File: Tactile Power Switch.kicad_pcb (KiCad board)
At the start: 2 copper layers, 24 x 30 mm, 16 parts, among them J1 OSTTC020162, J2 OSTTC020162, Q1 BC847B_215, Q2 BC847B_215, Q4 NDT2955

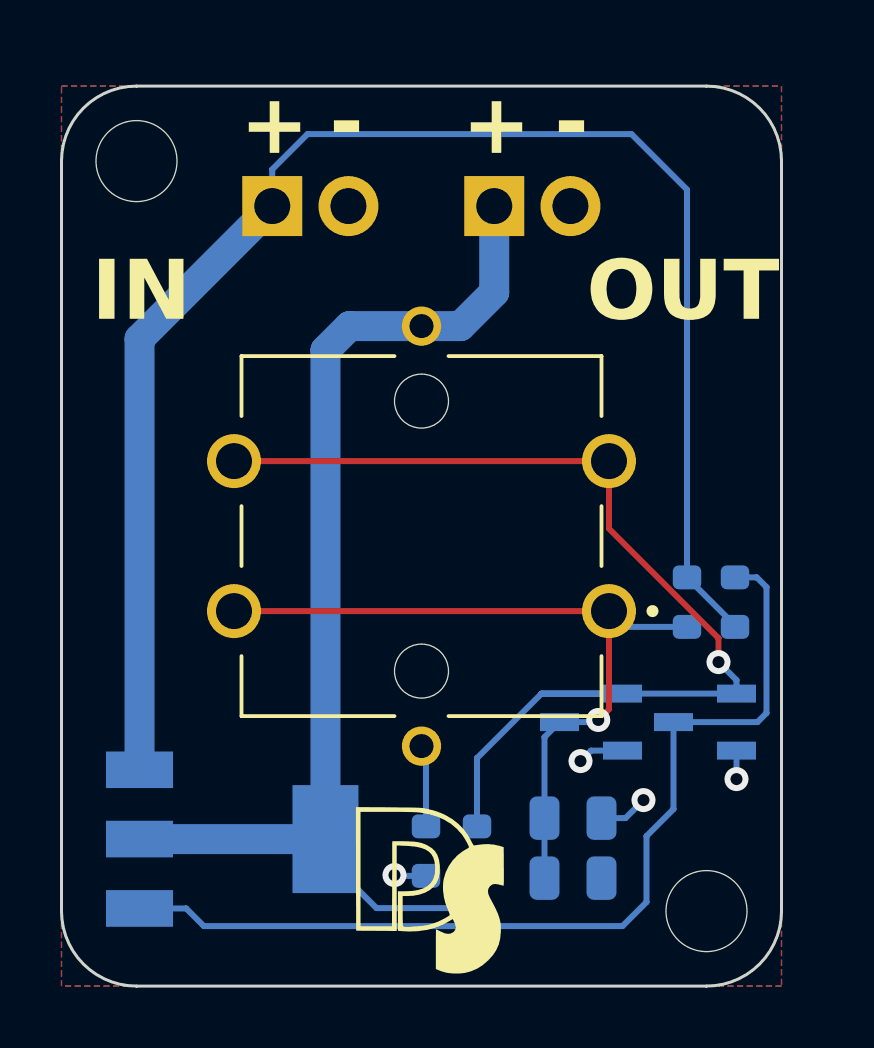
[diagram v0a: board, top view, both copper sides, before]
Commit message: SMD version: Placement is done
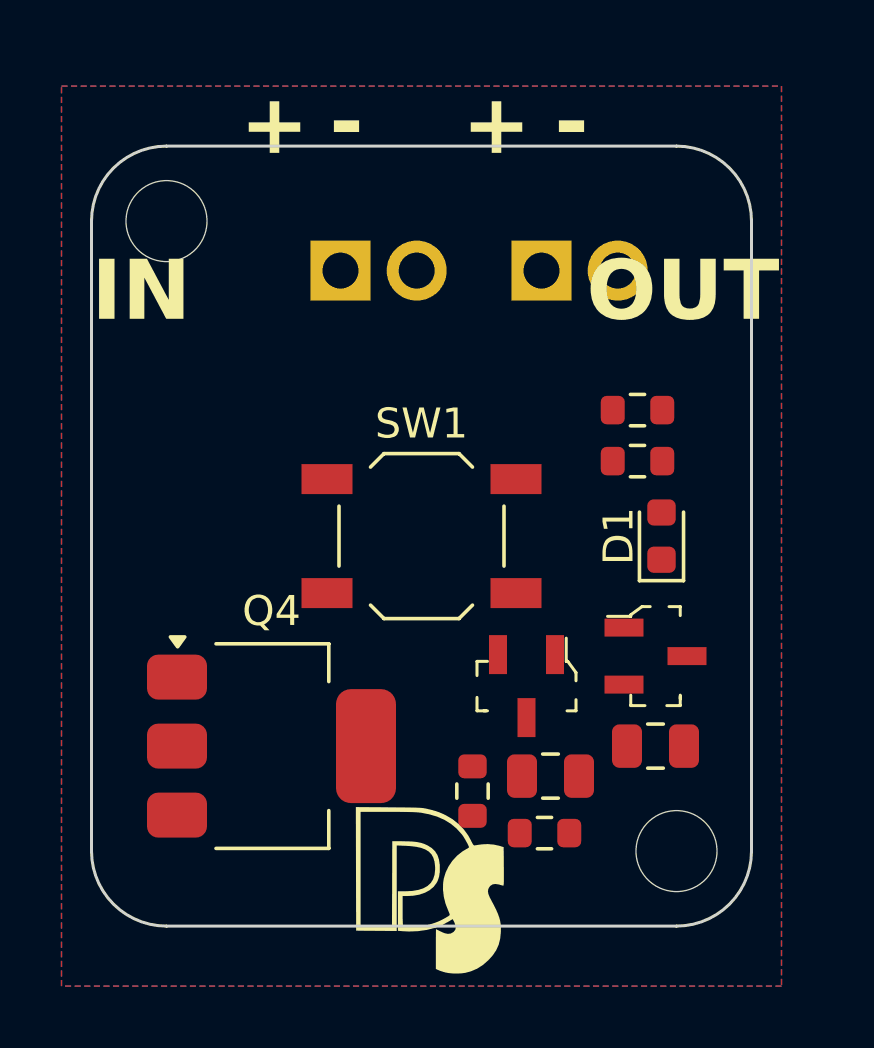
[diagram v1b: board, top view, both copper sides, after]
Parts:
- removed S1: TSD1265, SW_TSD1265:SW_TSD1265
- added D1: GREEN, LED_SMD:LED_0603_1608Metric, F.Cu at (128.0, 59.0)
- added SW1: SW_SPST, Button_Switch_SMD:SW_SPST_TL3342, F.Cu at (120.0, 59.0)
- C1, C2, Q1, Q2, R1, R2, R3, R4: moved to F.Cu
- Q4: footprint MOSFET:SOT223 -> Package_TO_SOT_SMD:SOT-223; moved to F.Cu
- moved R4 16.3 mm to (127.2, 54.8), turned to 180 degrees
- moved R2 14.1 mm to (127.2, 56.5), turned to 180 degrees
- moved R1 10.8 mm to (121.7, 67.5)
- moved R3 9.05 mm to (124.1, 68.9), turned to 0 degrees
- moved Q1 6.07 mm to (123.5, 64.0), turned to -90 degrees
- moved C1 3.65 mm to (127.8, 66.0)
- moved C2 3.48 mm to (124.3, 67.0), turned to 180 degrees
- moved Q4 3.36 mm to (115.0, 66.0), turned to 0 degrees
- moved J1 3.13 mm to (117.3, 50.1)
- moved Q2 3.08 mm to (127.8, 63.0), turned to 0 degrees
- moved J2 2.67 mm to (124.0, 50.1)
- moved H1 2.24 mm to (128.5, 69.5)
- moved H2 2.24 mm to (111.5, 48.5)
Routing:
- net +12V: track 52.2 -> 0.00 mm
- net VDD: track 39.1 -> 0.00 mm
- net Net-(Q1-B): track 36.5 -> 0.00 mm, vias 1 -> 0
- net Net-(Q1-C): track 32.5 -> 0.00 mm
- net Net-(Q2-C): track 25.8 -> 0.00 mm, vias 1 -> 0
- net GND: track 5.20 -> 0.00 mm, vias 4 -> 0
- net Net-(D1-K): track 2.74 -> 0.00 mm
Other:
- board size 24 x 30 mm -> 22 x 26 mm
